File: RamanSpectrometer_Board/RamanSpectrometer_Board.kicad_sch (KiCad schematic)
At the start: 35 parts, among them J1 RJ45_LED_Shielded, Q1 BSS138, Q2 BSS138, Q3 BSS138, Q4 BSS138, Q5 BSS138, U1 Teensy4.1_DEV-16771, U2 OKI 12V-5V, U3 OKI 5V-3V

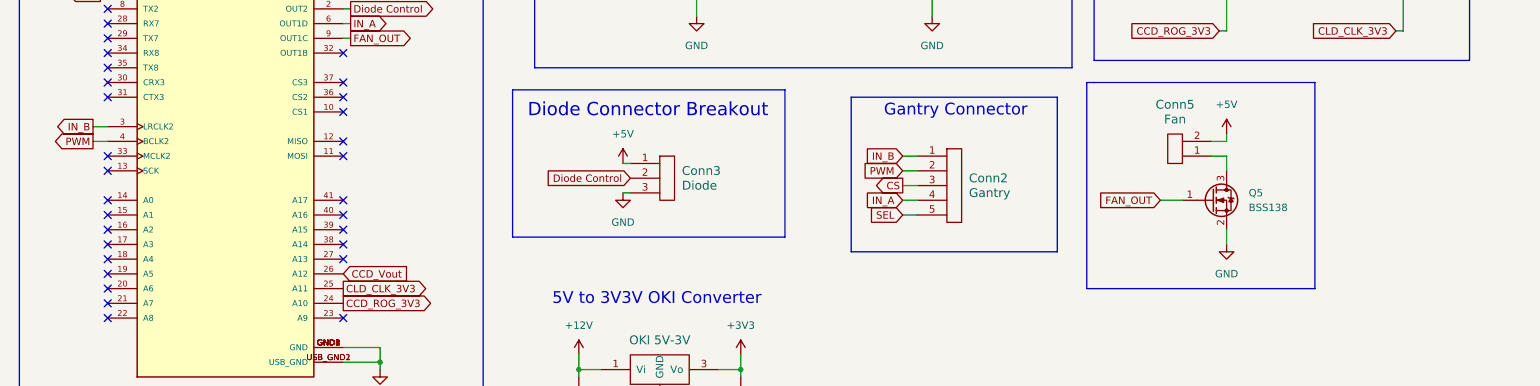
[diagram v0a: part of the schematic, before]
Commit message: PCB Raman edit and TOF
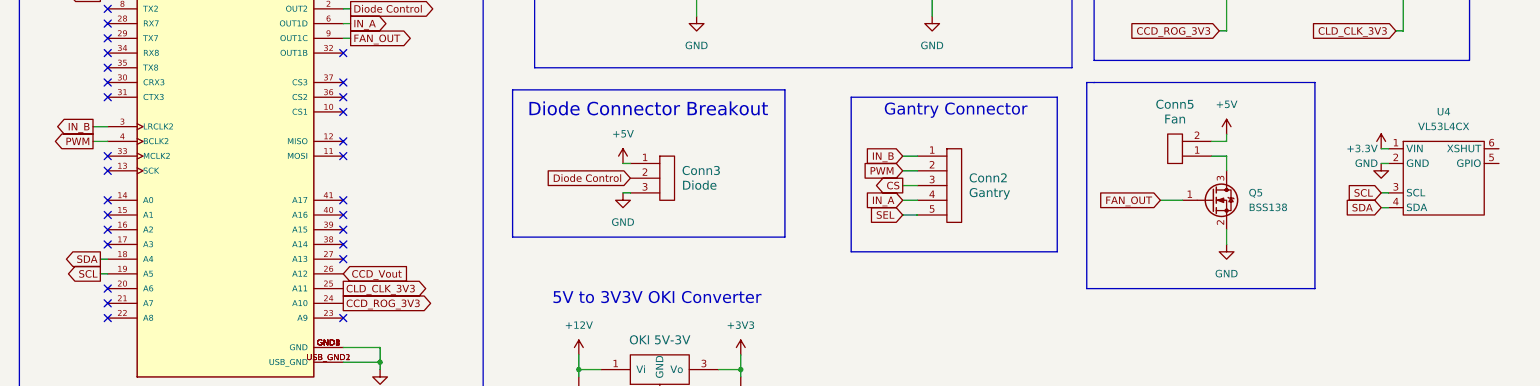
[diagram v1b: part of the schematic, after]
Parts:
- added U4: VL53L4CX, Connector_PinSocket_2.54mm:PinSocket_1x06_P2.54mm_Vertical, symbol MRDT_Sensors:VL53L4CX
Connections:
- net +3.3V: now also U4.1 (VIN)
- net GND: now also U4.2 (GND)
- net SDA: now reaches U1.18 (A4)
- net SDA: now also U4.4 (SDA)
- net SCL: now reaches U1.19 (A5)
- net SCL: now also U4.3 (SCL)
- no-connect marks 40 -> 38
